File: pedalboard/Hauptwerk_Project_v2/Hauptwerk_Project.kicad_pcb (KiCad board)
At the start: 2 copper layers, 233.7 x 49.5 mm, 50 parts, among them J1 Power 5V, J2 1-6, J3 7-12, J4 13-18, J5 19-24, J6 25-30, J7 31-32, U1 74HC165, U2 74HC165, U3 74HC165, U4 74HC165, U5 ProMicro

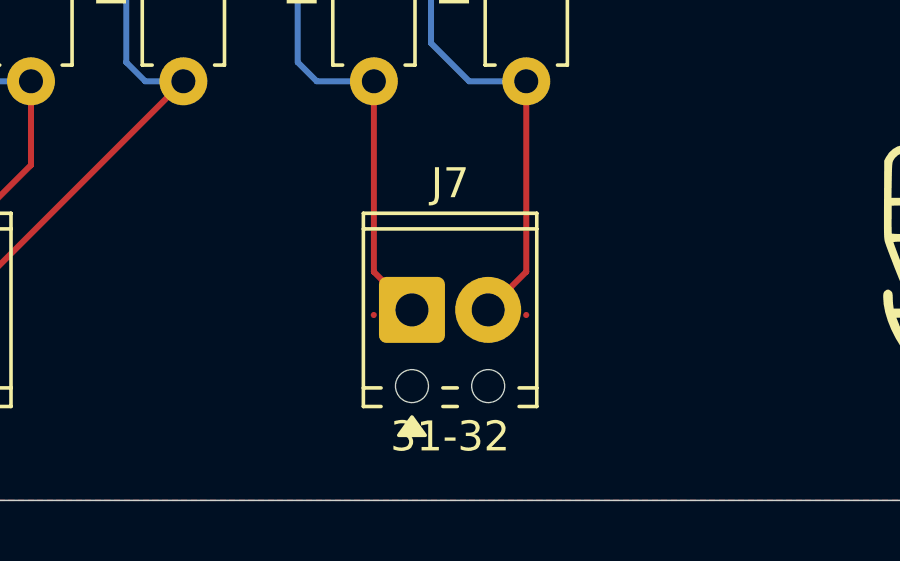
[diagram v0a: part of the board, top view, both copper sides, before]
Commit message: problem fix
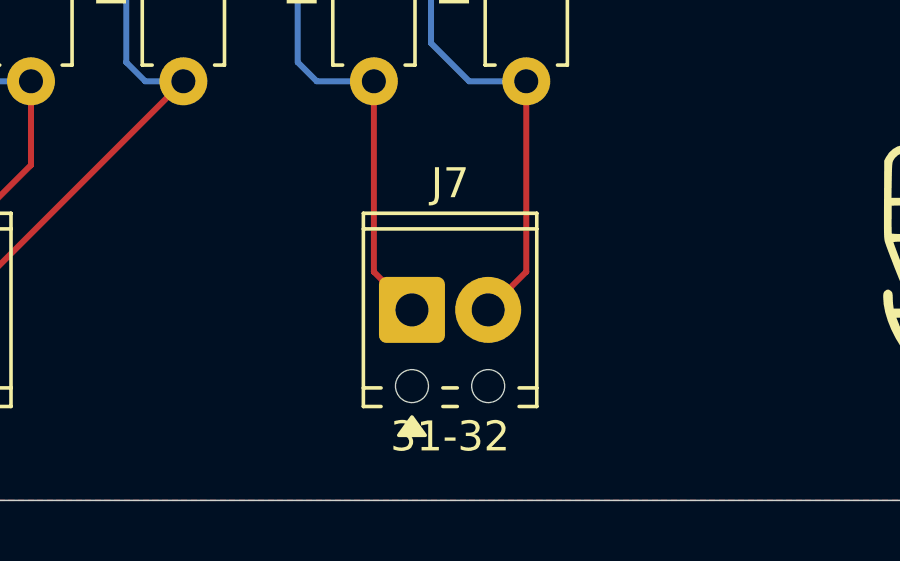
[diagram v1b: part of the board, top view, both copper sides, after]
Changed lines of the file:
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@@
-	)
-	(segment
-		(start 210.82 99.2275)
-		(end 210.815 99.2325)
-		(width 0.2)
-		(layer "F.Cu")
-		(net 33)
 	)
 	(segment
@@
 		(width 0.2)
 		(layer "F.Cu")
-		(net 34)
-	)
-	(segment
-		(start 205.74 99.2275)
-		(end 205.735 99.2325)
-		(width 0.2)
-		(layer "F.Cu")
